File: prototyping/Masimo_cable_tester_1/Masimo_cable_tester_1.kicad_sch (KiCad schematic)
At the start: 27 parts, among them J1 Touchscreen HMI, J12 Barrel_Jack, J16 Debug Connections, J17 Banana Jack, J18 Massimo Connector, J2 Conn_01x28_Socket, J3 Conn_01x28_Socket, J4 SD Card Reader, U1 J104D2C5VDC.15S, U2 LM7805_TO220

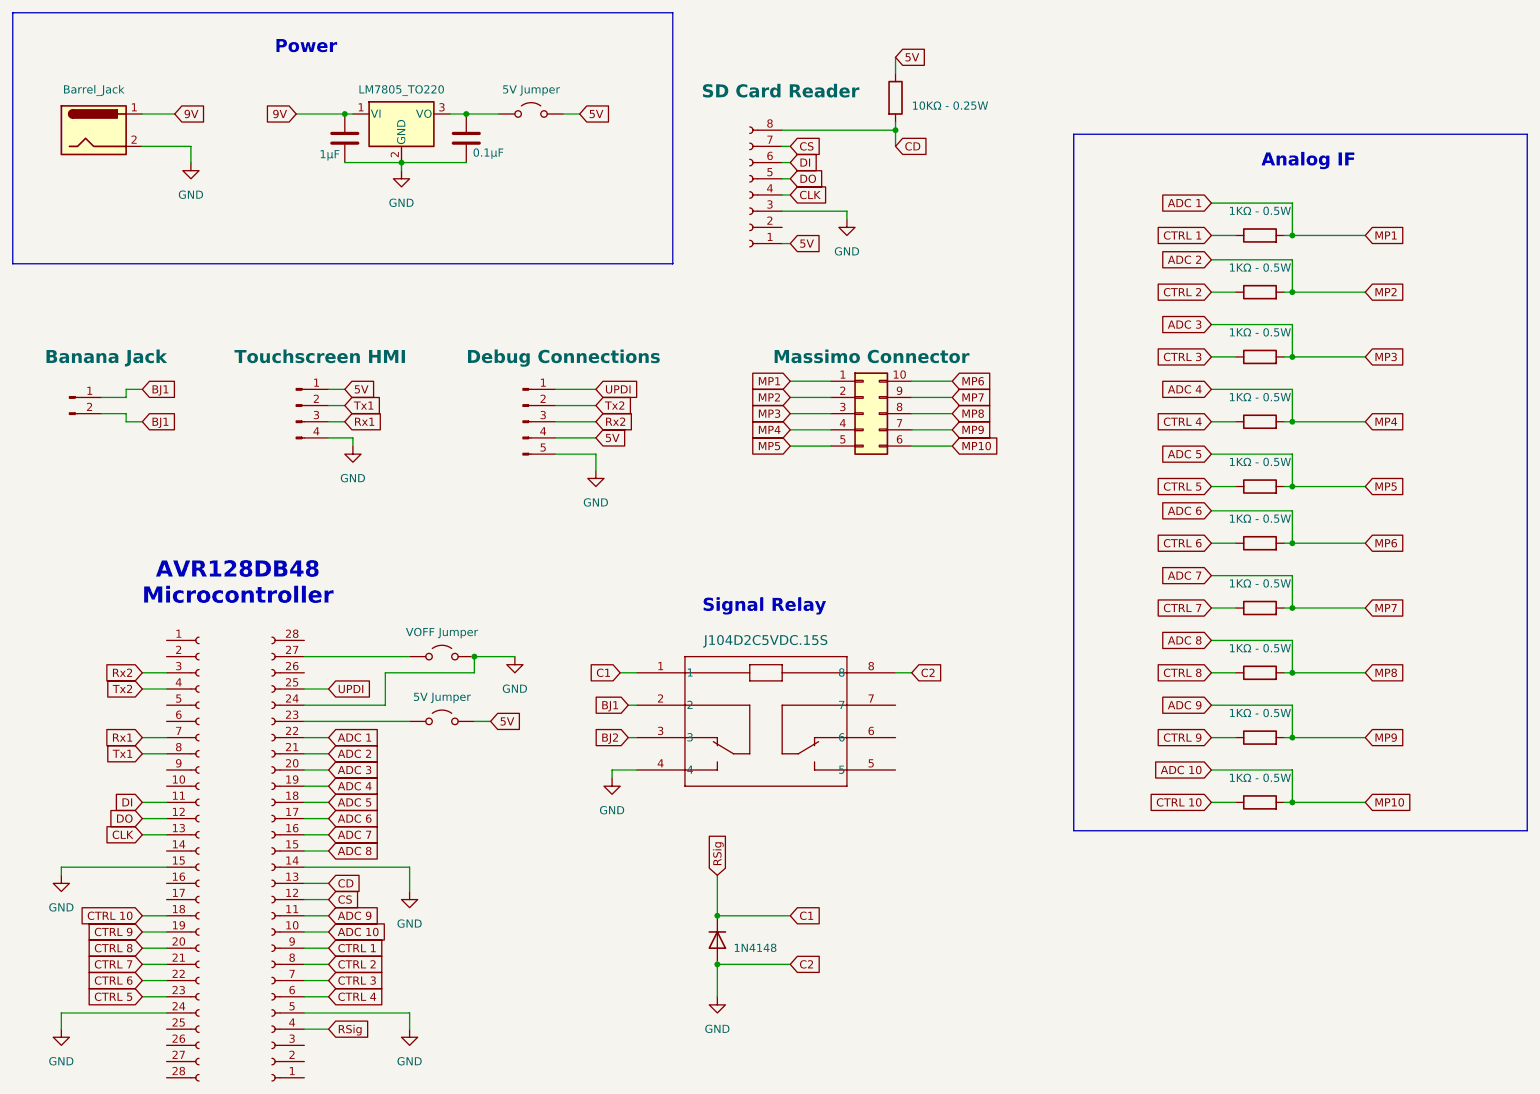
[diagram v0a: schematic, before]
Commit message: Prototype schematic updates
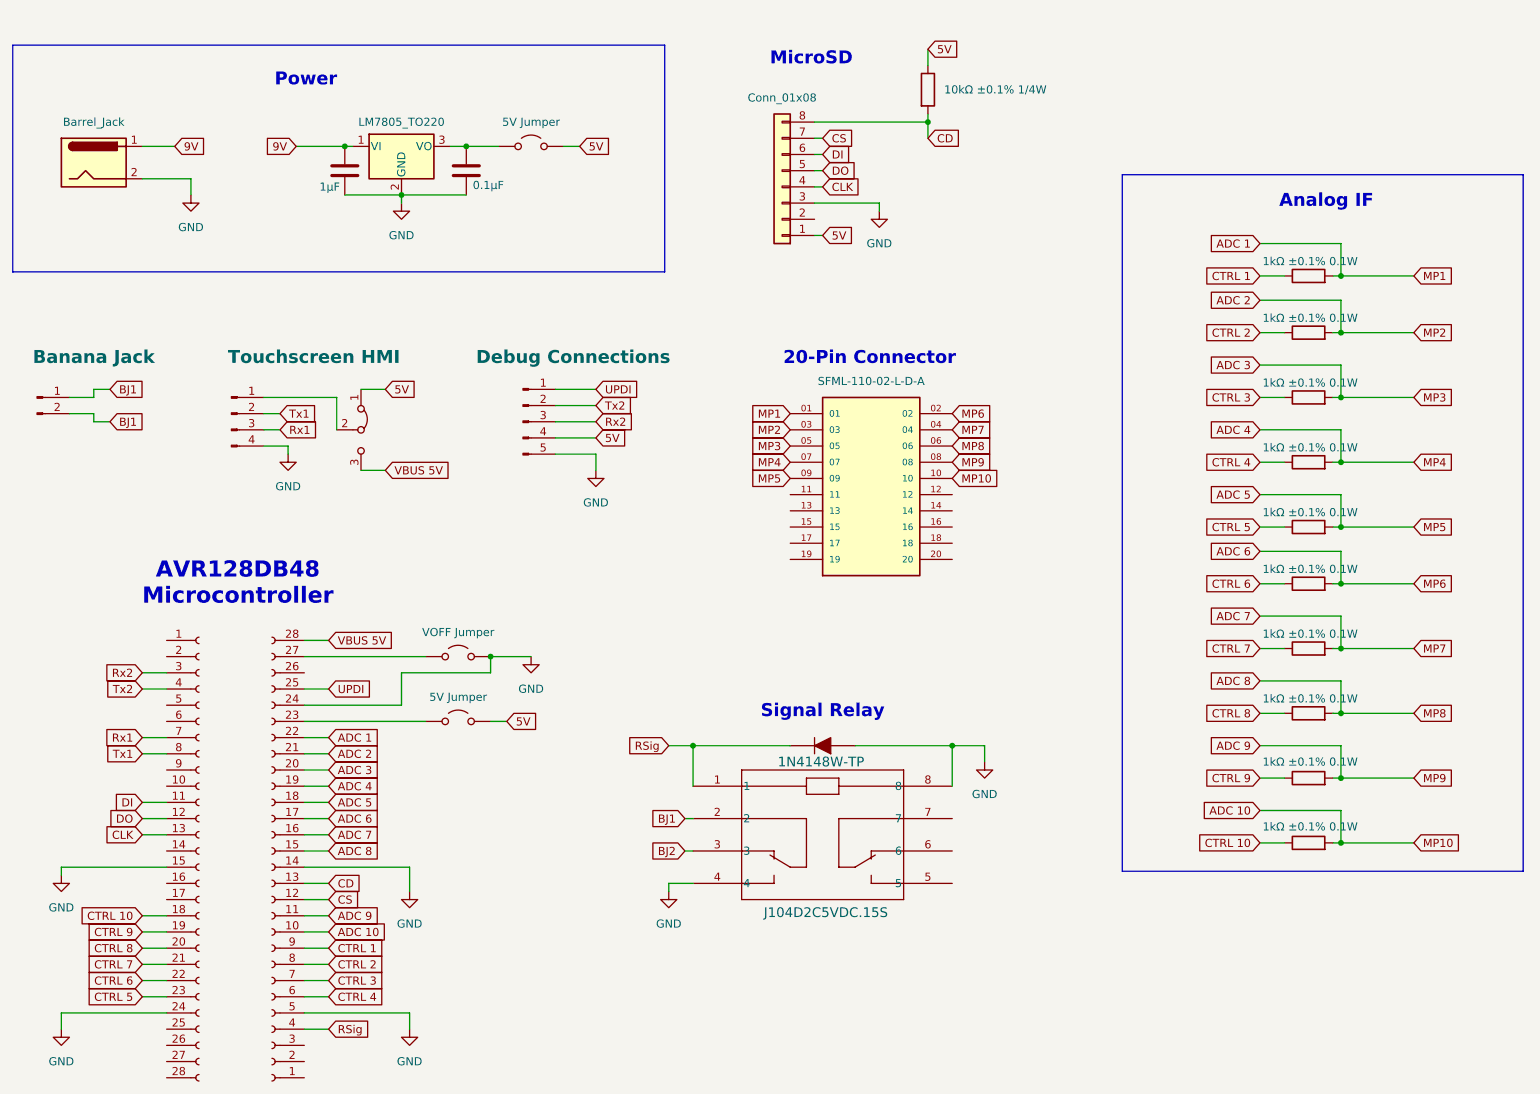
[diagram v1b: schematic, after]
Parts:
- removed D1: 1N4148, Diode_THT:D_DO-35_SOD27_P7.62mm_Horizontal, symbol Diode:1N4148
- removed J18: Massimo Connector, symbol Connector_Generic:Conn_02x05_Counter_Clockwise
- removed J4: SD Card Reader, Connector_PinSocket_1.00mm:PinSocket_1x08_P1.00mm_Vertical, symbol Connector:Conn_01x08_Socket
- added D2: 1N4148W-TP, digikey-footprints:SOD-123, symbol dk_Diodes-Rectifiers-Single:1N4148W-TP
- added J5: Conn_01x08, Connector_PinHeader_2.54mm:PinHeader_1x08_P2.54mm_Vertical, symbol Connector_Generic:Conn_01x08
- added J6: SFML-110-02-L-D-A, SFML_110_02_L_D_A:SAMTEC_SFML-110-02-L-D-A, symbol SFML-110-02-L-D-A:SFML-110-02-L-D-A
- added JP4: HMI Power Jumper, symbol Jumper:Jumper_3_Bridged12
- J1: footprint (none) -> Connector_PinHeader_2.54mm:PinHeader_1x04_P2.54mm_Vertical
- J16: footprint (none) -> Connector_PinHeader_2.54mm:PinHeader_1x05_P2.54mm_Vertical
- J17: footprint (none) -> Connector_PinHeader_2.54mm:PinHeader_1x02_P2.54mm_Vertical
- R1: value 10KΩ - 0.25W -> 10kΩ ±0.1% 1/4W
- R10, R11, R12, R3, R4, R5, R6, R7, R8, R9: value 1KΩ - 0.5W -> 1kΩ ±0.1% 0.1W
- U1: footprint RELAY8_J104D2C5VDC.20S_CRS -> footprints:RELAY8_J104D2C5VDC.20S_CRS
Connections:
- net 5V: now also J5.1 (Pin_1), JP4.1 (A); no longer J1.1 (Pin_1)
- net ADC 1: now also J6.01
- net ADC 10: now also J6.10
- net ADC 2: now also J6.03
- net ADC 3: now also J6.05
- net ADC 4: now also J6.07
- net ADC 5: now also J6.09
- net ADC 6: now also J6.02
- net ADC 7: now also J6.04
- net ADC 8: now also J6.06
- net ADC 9: now also J6.08
- net CD: now also J5.8 (Pin_8)
- net CLK: now also J5.4 (Pin_4)
- net CS: now also J5.7 (Pin_7)
- net DI: now also J5.6 (Pin_6)
- net DO: now also J5.5 (Pin_5)
- net GND: now also D2.A, J5.3 (Pin_3)
- net VBUS 5V: now reaches J3.28 (Pin_28)
- net VBUS 5V: now also JP4.3 (B)
- net C1 renamed RSig
- net RSig: now also D2.K
- new net: J1.1 (Pin_1), JP4.2 (C)
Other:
- note added: "20-Pin Connector"
- note added: "MicroSD"
- company: SDSU Senior Design A -> SDSU Senior Design B
- title: Masimo Cable Tester -> Automated multiconductor cable break-short detector
